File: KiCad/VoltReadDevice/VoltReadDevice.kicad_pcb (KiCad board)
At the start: 2 copper layers, 48.3 x 39.4 mm, 6 parts, among them J1 Conn_PinHeader_1x04_P2.54mm_H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, J2 Conn_PinHeader_1x04_P2.54mm_H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, J3 Conn_PinHeader_1x02_P2.54mm_H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, U1 ATtiny412-SS

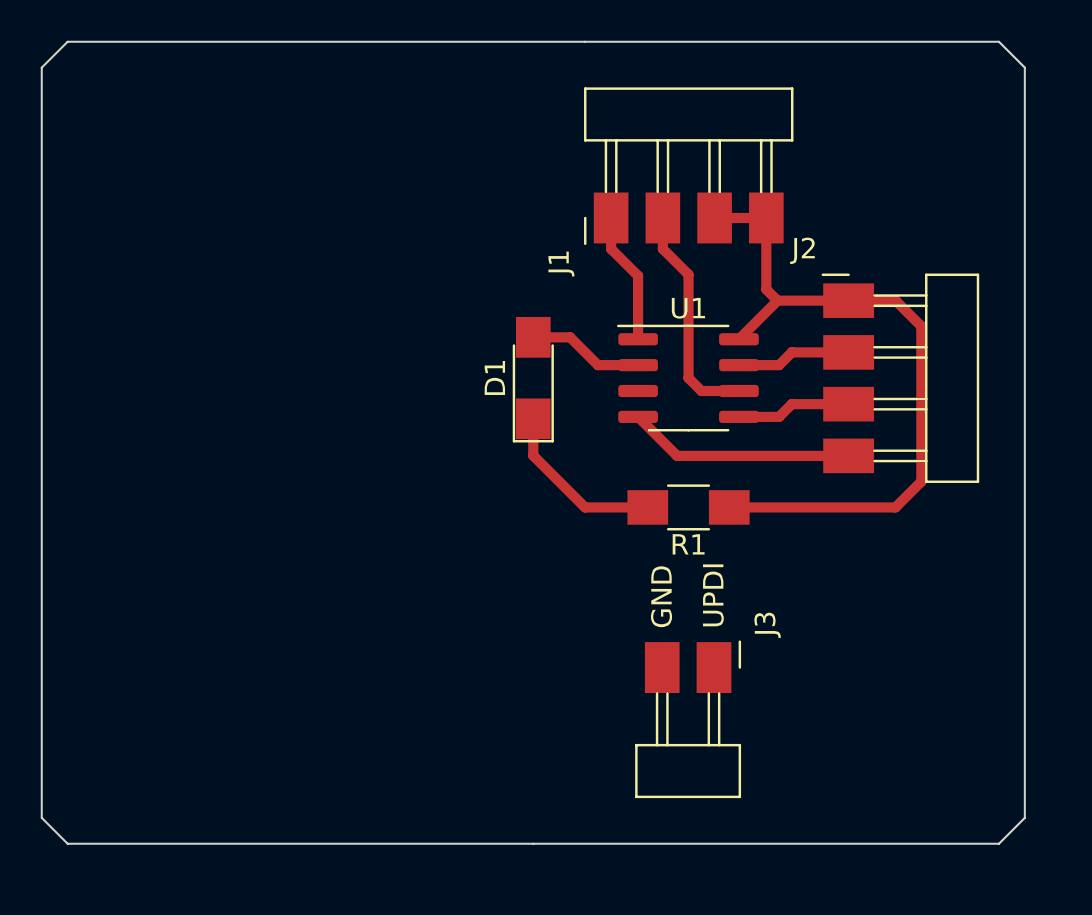
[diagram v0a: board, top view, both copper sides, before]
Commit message: v2.4 - Finished KiCad Design
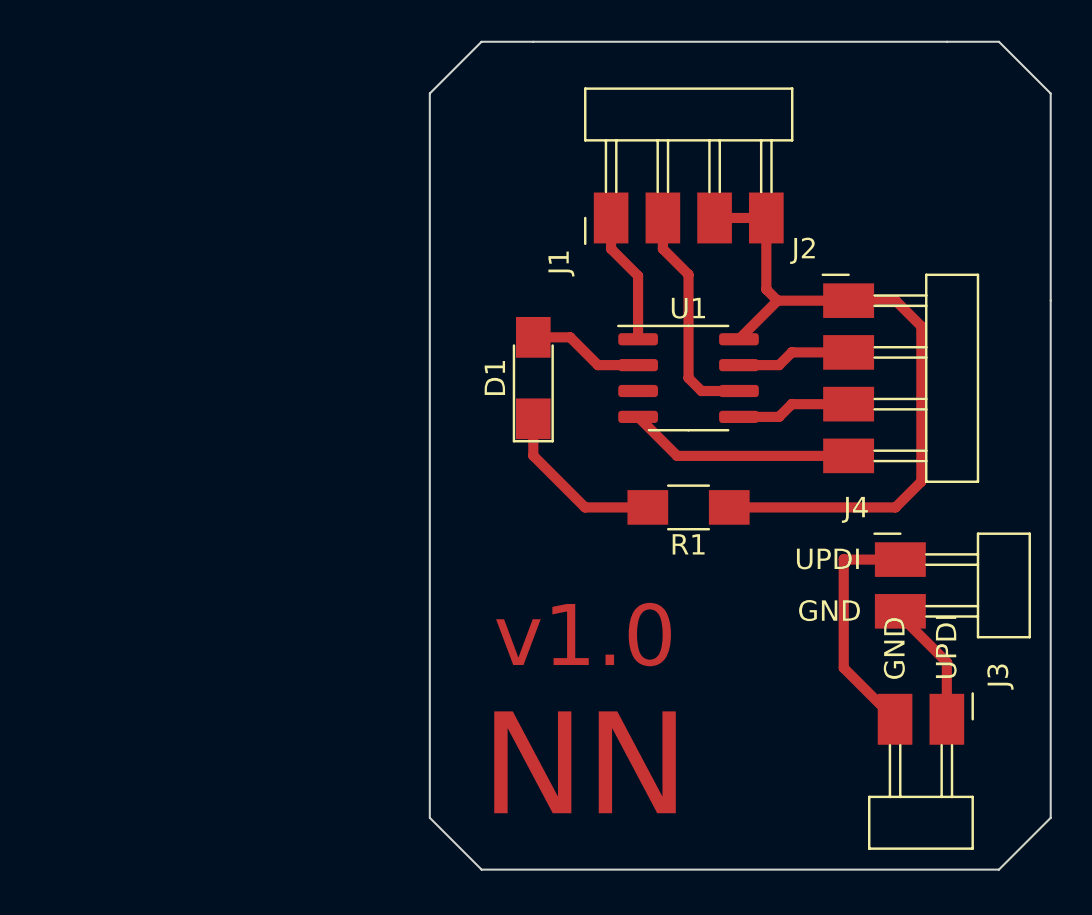
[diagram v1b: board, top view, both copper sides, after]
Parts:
- added J4: Conn_PinHeader_1x02_P2.54mm_Horizontal_SMD, fab:PinHeader_UPDI_01x02_P2.54mm_Horizontal_SMD, F.Cu at (175.5, 124.5)
- moved J3 11.7 mm to (177.8, 132.3)
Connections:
- J3 pad 1: unconnected-(J3-Pad1) -> Net-(J3-Pad1)
- J3 pad 2: unconnected-(J3-Pad2) -> Net-(J3-Pad2)
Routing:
- net Net-(J3-Pad2): track 0.00 -> 11.7 mm
- net Net-(J3-Pad1): track 0.00 -> 6.26 mm
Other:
- board size 48.3 x 39.4 mm -> 30.5 x 40.6 mm
- board text added: "NN"
- board text added: "v1.0"
